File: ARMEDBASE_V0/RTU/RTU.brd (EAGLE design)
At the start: 99 x 69.5 mm, 27 parts, among them IC1 REG1117, IC2 MEGA8-P, Q1 20Mhz, Q2 2N3904

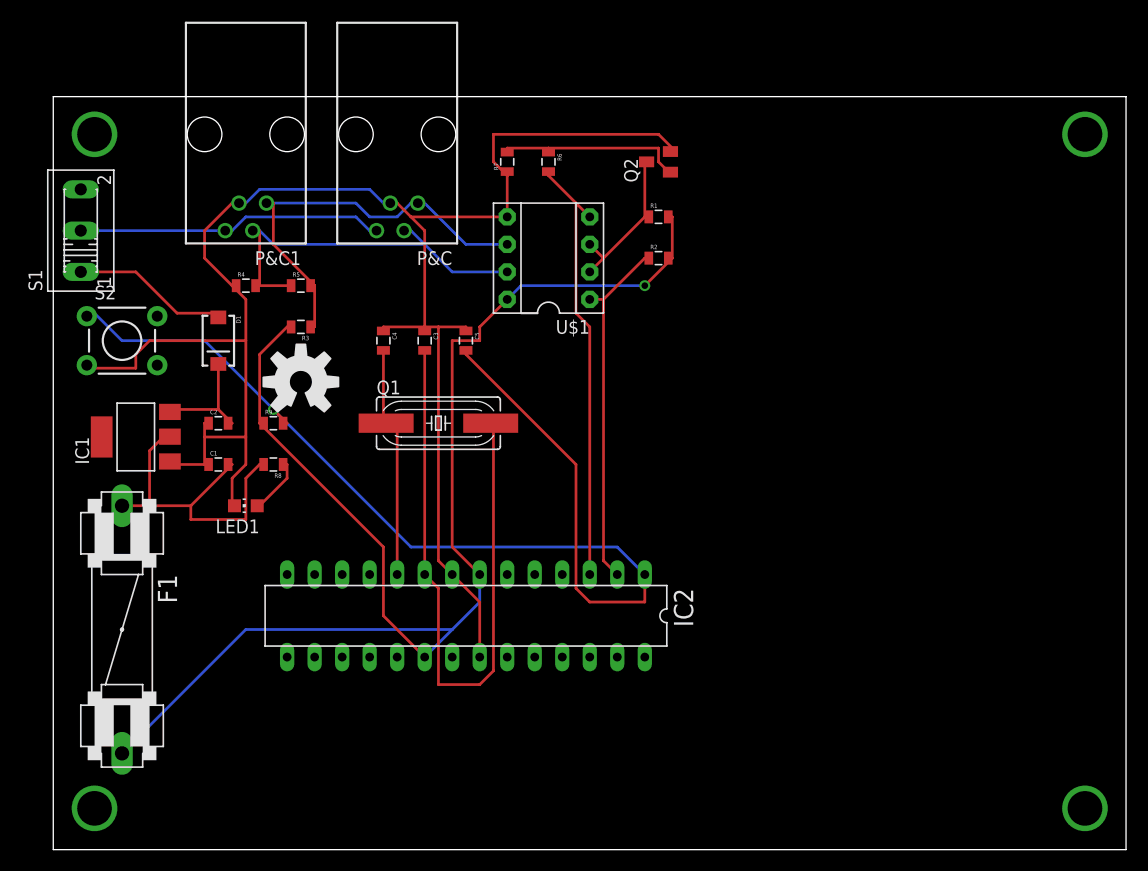
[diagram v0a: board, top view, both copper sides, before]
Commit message: rtu fuse
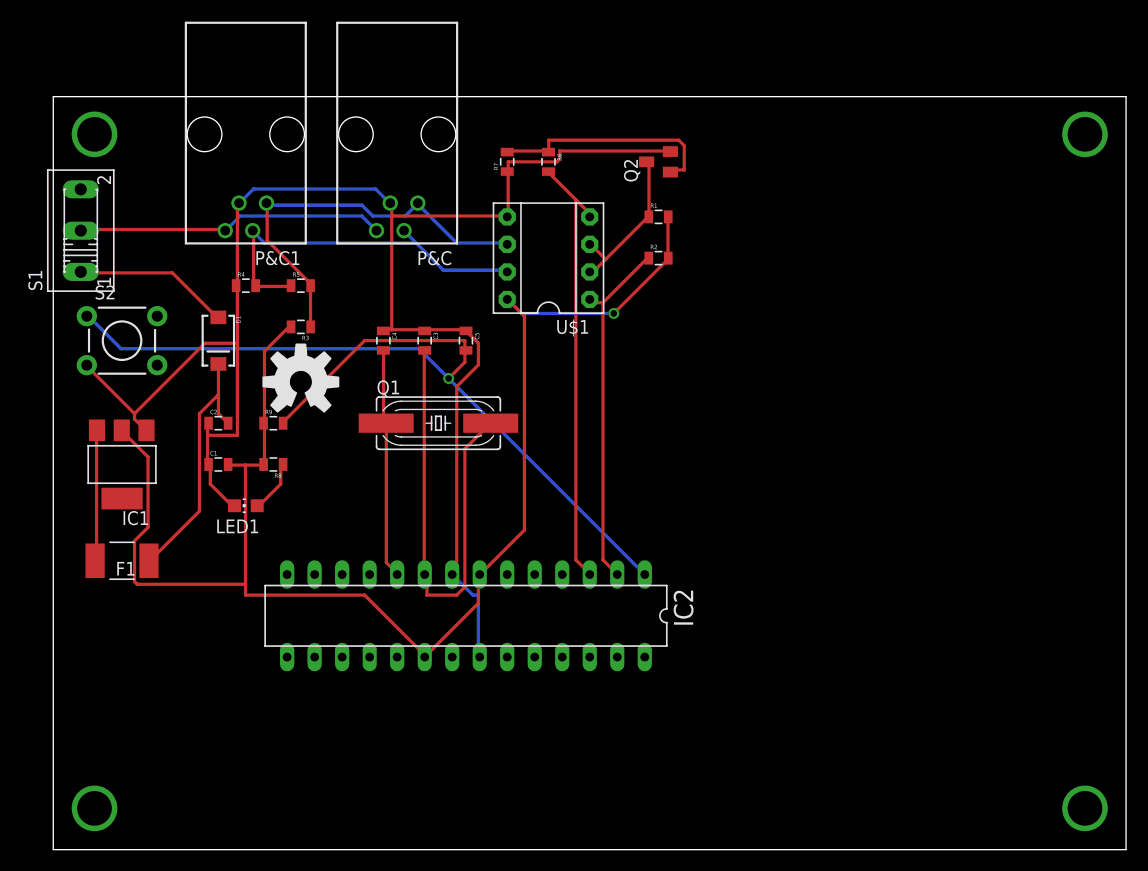
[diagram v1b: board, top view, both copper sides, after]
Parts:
- F1: value 100mA -> 100ma; device special:FUSE -> _hhn_PtcFuses_Siba_r500_Ozan:1820
- moved F1 6.35 mm to (6.35, 26.7), turned to 180 degrees
- moved IC1 2.84 mm to (6.35, 35.6), turned to 180 degrees
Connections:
- net N$9: now also F1.2, IC1.3; no longer C1.2, F1.1, IC1.2, R8.2
- net VCC12V: now also F1.1; no longer IC1.3
- net VCC5V: now also C1.2, IC1.2, R8.2; no longer F1.2
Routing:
- net N$9: track 31.9 -> 12.1 mm
- net N$21: track 60.1 -> 42.6 mm
- net N$24: track 99.3 -> 85.6 mm
- net VCC12V: track 10.9 -> 23.9 mm
- net GND: track 164.2 -> 153.1 mm
- net N$4: track 18.1 -> 21.4 mm
- net VCC5V: track 134.9 -> 132.9 mm
- net N$7: track 36.5 -> 35.2 mm
- net N$8: track 39.2 -> 38.0 mm
- net N$23: track 22.0 -> 21.2 mm
